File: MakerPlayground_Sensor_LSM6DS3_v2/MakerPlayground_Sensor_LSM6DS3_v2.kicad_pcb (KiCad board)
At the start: 2 copper layers, 30.4 x 19.9 mm, 16 parts, among them J1 Conn_01x04, Q1 BSS138, Q2 BSS138, U1 AP2127K-3.3, U2 LSM6DS3

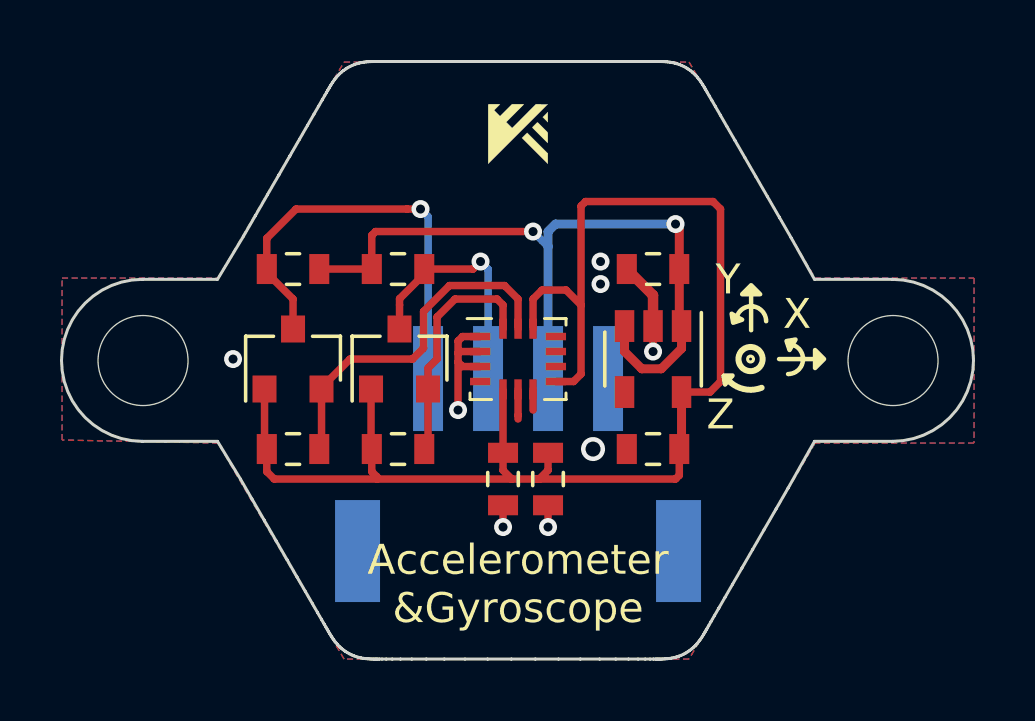
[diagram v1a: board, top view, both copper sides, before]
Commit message: Complete design.
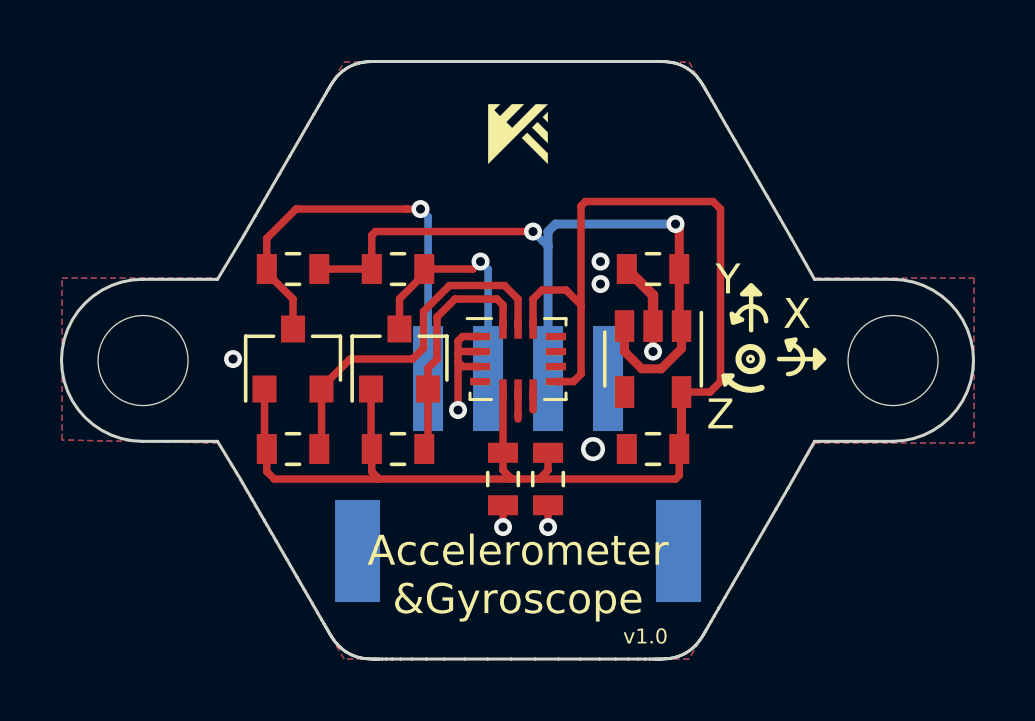
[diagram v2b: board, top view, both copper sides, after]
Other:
- board text added: "v1.0"
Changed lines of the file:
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@@
   (general
     (thickness 1.6)
-    (drawings 238)
+    (drawings 239)
     (tracks 122)
     (zones 0)
@@
     (46 B.CrtYd user)
     (47 F.CrtYd user)
-    (48 B.Fab user)
-    (49 F.Fab user)
+    (48 B.Fab user hide)
+    (49 F.Fab user hide)
   )
   (setup
@@
     )
     (pad 1 np_thru_hole circle (at 0 0) (size 3 3) (drill 3) (layers *.Cu *.Mask))
+  )
+  (gr_text v1.0 (at 150.75 109.25) (layer F.SilkS)
+    (effects (font (size 0.5 0.5) (thickness 0.1)))
   )
   (gr_line (start 141.686 110) (end 141.734 110) (layer Edge.Cuts) (width 0.1))
@@
   )
   (gr_line (start 155.2 100) (end 156.6 100) (layer F.SilkS) (width 0.15))
-  (gr_text "Accelerometer\n&Gyroscope" (at 146.5 107.5) (layer F.SilkS)
+  (gr_text "Accelerometer\n&Gyroscope" (at 146.5 107.2) (layer F.SilkS)
     (effects (font (size 1 1) (thickness 0.2)))
   )
